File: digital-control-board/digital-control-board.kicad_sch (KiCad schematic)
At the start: 0 parts

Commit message: Get some design from rp minimal board
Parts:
- added C1, C19, C5: 10u, Capacitor_SMD:C_0805_2012Metric, symbol Device:C
- added C10, C9: 4.7u, Capacitor_SMD:C_0402_1005Metric, symbol Device:C
- added C11, C12, C13, C14, C15, C16, C17, C18, C2, C20, C21, C8: 100n, Capacitor_SMD:C_0402_1005Metric, symbol Device:C
- added C22: DNF, Capacitor_SMD:C_0402_1005Metric, symbol Device:C
- added C3, C4: 15p, Capacitor_SMD:C_0402_1005Metric, symbol Device:C
- added C6, C7: 4.7u, RP2350_80QFN_minimal:C_0402_1005Metric_small_pads, symbol Device:C
- added DN1: PM127-2-10-S-4.3, programmable-load-library:HDR-SMD_20P-P1.27-V-F-R2-C10-LS4.8, symbol programmable-load-library:PM127-2-10-S-4.3
- added J1: USB_B_Micro, Connector_USB:USB_Micro-B_Amphenol_10103594-0001LF_Horizontal, symbol Connector:USB_B_Micro
- added J4: SM03B-SRSS-TB, Connector_JST:JST_SH_SM03B-SRSS-TB_1x03-1MP_P1.00mm_Horizontal, symbol Connector_Generic_MountingPin:Conn_01x03_MountingPin
- added L1: 3.3u, RP2350_80QFN_minimal:L_pol_2016, symbol Device:L
- added R1, R11, R13, R9: DNF, Resistor_SMD:R_0402_1005Metric, symbol Device:R
- added R10: 0, Resistor_SMD:R_0402_1005Metric, symbol Device:R
- added R2, R4, R6: 1k, Resistor_SMD:R_0402_1005Metric, symbol Device:R
- added R3: 33, Resistor_SMD:R_0402_1005Metric, symbol Device:R
- added R7, R8: 27, Resistor_SMD:R_0402_1005Metric, symbol Device:R
- added SW1, SW2: SW_Push, Button_Switch_SMD:SW_Push_1P1T_NO_Vertical_Wuerth_434133025816, symbol Switch:SW_Push
- added U1: RP2350_80QFN, RP2350_80QFN_minimal:RP2350-QFN-80-1EP_10x10_P0.4mm_EP3.4x3.4mm_ThermalVias, symbol MCU_RaspberryPi_RP2350:RP2350_80QFN
- added U2: NCP1117-3.3_SOT223, Package_TO_SOT_SMD:SOT-223-3_TabPin2, symbol Regulator_Linear:NCP1117-3.3_SOT223
- added U3: W25Q128JVS, Package_SO:SOIC-8_5.23x5.23mm_P1.27mm, symbol Memory_Flash:W25Q128JVS
- added U4: DNF, Package_SO:SOIC-8_5.23x5.23mm_P1.27mm, symbol Memory_Flash:W25Q128JVS
- added Y1: ABM8-272-T3, Crystal:Crystal_SMD_3225-4Pin_3.2x2.5mm, symbol Device:Crystal_GND24
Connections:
- new net: C4.1, R2.2, Y1.3
- new net: R7.2, U1.67 (USB_DP)
- new net: R8.2, U1.66 (USB_DM)
- new net: R4.1, SW2.1
- new net +1V1: C10.1, C11.1, C7.1, C8.1, L1.1, U1.10 (DVDD), U1.32 (DVDD), U1.51 (DVDD), U1.65 (VREG_FB)
- new net +3V3: C12.1, C13.1, C14.1, C15.1, C16.1, C17.1, C18.1, C19.1, C2.1, C20.1, C21.1, C22.1, C5.1, C6.1, R1.1, R13.1, R3.1, U1.15 (IOVDD), U1.24 (IOVDD), U1.29 (IOVDD), U1.41 (IOVDD), U1.5 (IOVDD), U1.50 (IOVDD), U1.59 (ADC_AVDD), U1.60 (IOVDD), U1.64 (VREG_VIN), U1.68 (USB_OTP_VDD), U1.69 (QSPI_IOVDD), U1.76 (IOVDD), U2.2 (VO), U3.8 (VCC), U4.8 (VCC)
- new net FLASH2_SS: R11.2, R13.2, U4.1 (~{CS})
- new net FLASH_SS: R1.2, R10.2, R9.2, U3.1 (~{CS})
- new net GND: C1.2, C10.2, C11.2, C12.2, C13.2, C14.2, C15.2, C16.2, C17.2, C18.2, C19.2, C2.2, C20.2, C21.2, C22.2, C3.2, C4.2, C5.2, C6.2, C7.2, C8.2, C9.2, J1.5 (GND), J1.6 (Shield), J4.2 (Pin_2), J4.MP (MountPin), R4.2, SW1.1, U1.62 (VREG_PGND), U1.81 (GND), U2.1 (GND), U3.4 (GND), U4.4 (GND), Y1.2, Y1.4
- new net GPIO0: R11.1, U1.77 (GPIO0)
- new net GPIO1: U1.78 (GPIO1)
- new net GPIO10: U1.8 (GPIO10)
- new net GPIO11: U1.9 (GPIO11)
- new net GPIO12: U1.11 (GPIO12)
- new net GPIO13: U1.12 (GPIO13)
- new net GPIO14: U1.13 (GPIO14)
- new net GPIO15: U1.14 (GPIO15)
- new net GPIO16: U1.16 (GPIO16)
- new net GPIO17: U1.17 (GPIO17)
- new net GPIO18: U1.18 (GPIO18)
- new net GPIO19: U1.19 (GPIO19)
- new net GPIO2: U1.79 (GPIO2)
- new net GPIO20: U1.20 (GPIO20)
- new net GPIO21: U1.21 (GPIO21)
- new net GPIO22: U1.22 (GPIO22)
- new net GPIO23: U1.23 (GPIO23)
- new net GPIO24: U1.25 (GPIO24)
- new net GPIO25: U1.26 (GPIO25)
- new net GPIO26: U1.27 (GPIO26)
- new net GPIO27: U1.28 (GPIO27)
- new net GPIO28: U1.36 (GPIO28)
- new net GPIO29: U1.37 (GPIO29)
- new net GPIO3: U1.80 (GPIO3)
- new net GPIO30: U1.38 (GPIO30)
- new net GPIO31: U1.39 (GPIO31)
- new net GPIO32: U1.40 (GPIO32)
- new net GPIO33: U1.42 (GPIO33)
- new net GPIO34: U1.43 (GPIO34)
- new net GPIO35: U1.44 (GPIO35)
- new net GPIO36: U1.45 (GPIO36)
- new net GPIO37: U1.46 (GPIO37)
- new net GPIO38: U1.47 (GPIO38)
- new net GPIO39: U1.48 (GPIO39)
- new net GPIO4: U1.1 (GPIO4)
- new net GPIO40_ADC0: U1.49 (GPIO40_ADC0)
- new net GPIO41_ADC1: U1.52 (GPIO41_ADC1)
- new net GPIO42_ADC2: U1.53 (GPIO42_ADC2)
- new net GPIO43_ADC3: U1.54 (GPIO43_ADC3)
- new net GPIO44_ADC4: U1.55 (GPIO44_ADC4)
- new net GPIO45_ADC5: U1.56 (GPIO45_ADC5)
- new net GPIO46_ADC6: U1.57 (GPIO46_ADC6)
- new net GPIO47_ADC7: U1.58 (GPIO47_ADC7)
- new net GPIO5: U1.2 (GPIO5)
- new net GPIO6: U1.3 (GPIO6)
- new net GPIO7: U1.4 (GPIO7)
- new net GPIO8: U1.6 (GPIO8)
- new net GPIO9: U1.7 (GPIO9)
- new net QSPI_SCLK: U1.71 (QSPI_SCLK), U3.6 (CLK), U4.6 (CLK)
- new net QSPI_SD0: U1.72 (QSPI_SD0), U3.5 (DI(IO0)), U4.5 (DI(IO0))
- new net QSPI_SD1: U1.74 (QSPI_SD1), U3.2 (DO(IO1)), U4.2 (DO(IO1))
- new net QSPI_SD2: U1.73 (QSPI_SD2), U3.3 (IO2), U4.3 (IO2)
- new net QSPI_SD3: U1.70 (QSPI_SD3), U3.7 (IO3), U4.7 (IO3)
- new net QSPI_SS: R6.1, U1.75 (QSPI_SS)
- new net RUN: SW2.2, U1.35 (RUN)
- new net SWCLK: J4.1 (Pin_1), U1.33 (SWCLK)
- new net SWD: J4.3 (Pin_3), U1.34 (SWD)
- new net USB_D+: J1.3 (D+), R7.1
- new net USB_D-: J1.2 (D-), R8.1
- new net VBUS: C1.1, J1.1 (VBUS), U2.3 (VI)
- new net VREG_AVDD: C9.1, R3.2, U1.61 (VREG_AVDD)
- new net VREG_LX: L1.2, U1.63 (VREG_LX)
- new net XIN: C3.1, U1.30 (XIN), Y1.1
- new net XOUT: R2.1, U1.31 (XOUT)
- new net ~{USB_BOOT}: R6.2, SW1.2
- no-connect marks 0 -> 1
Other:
- note added: "12MHz Crystal"
- note added: "JST Debug Connector"
- note added: "Make sure R7 and R8 are close to RP2350"
- note added: "Optional Secondary flash or PSRAM (U4), using the second chip select (XIP_SS_N[1]) on GPIO0. N.B. Pull-up R13 will be required as GPIOs default to pull-downs at power-up."
- note added: "Power"
- note added: "Primary Flash"
- note added: "Reference the RP2350 minimal design example caz I'm lazy"
- note added: "Secondary Flash/PSRAM"

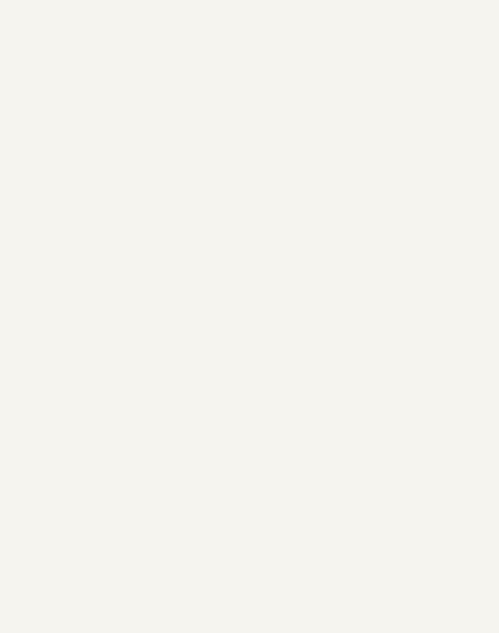
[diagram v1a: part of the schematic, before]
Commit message: Update sch
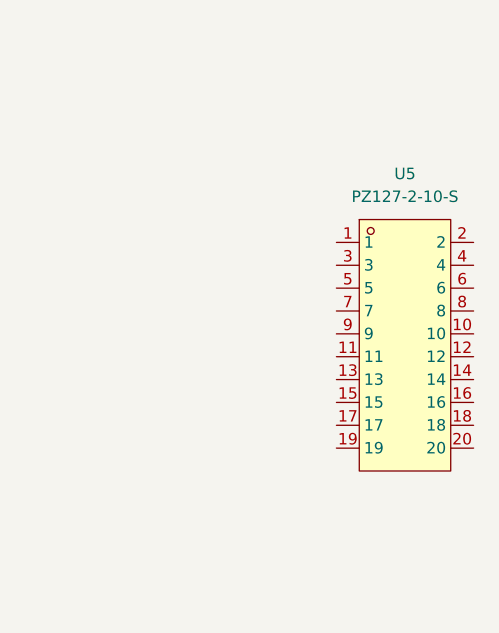
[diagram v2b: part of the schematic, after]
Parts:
- added U5: PZ127-2-10-S, programmable-load-library:HDR-SMD_PZ127-2-10-S, symbol programmable-load-library:PZ127-2-10-S
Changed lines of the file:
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@@
+	)
+	(symbol
+		(lib_id "programmable-load-library:PZ127-2-10-S")
+		(at 519.43 64.77 0)
+		(unit 1)
+		(exclude_from_sim no)
+		(in_bom yes)
+		(on_board yes)
+		(dnp no)
+		(fields_autoplaced yes)
+		(property "Reference" "U5"
+			(at 519.43 45.72 0)
+			(effects
+				(font
+					(size 1.27 1.27)
+				)
+			)
+		)
+		(property "Value" "PZ127-2-10-S"
+			(at 519.43 48.26 0)
+			(effects
+				(font
+					(size 1.27 1.27)
+				)
+			)
+		)
+		(property "Footprint" "programmable-load-library:HDR-SMD_PZ127-2-10-S"
+			(at 519.43 83.82 0)
+			(effects
+				(font
+					(size 1.27 1.27)
+				)
+				(hide yes)
+			)
+		)
+		(property "Datasheet" ""
+			(at 519.43 64.77 0)
+			(effects
+				(font
+					(size 1.27 1.27)
+				)
+				(hide yes)
+			)
+		)
+		(property "Description" ""
+			(at 519.43 64.77 0)
+			(effects
+				(font
+					(size 1.27 1.27)
+				)
+				(hide yes)
+			)
+		)
+		(property "LCSC Part" "C3975193"
+			(at 519.43 86.36 0)
+			(effects
+				(font
+					(size 1.27 1.27)
+				)
+				(hide yes)
+			)
+		)
+		(pin "19"
+		)
+		(pin "2"
+		)
+		(pin "4"
+		)
+		(pin "6"
+		)
+		(pin "8"
+		)
+		(pin "10"
+		)
+		(pin "12"
+		)
+		(pin "14"
+		)
+		(pin "16"
+		)
+		(pin "18"
+		)
+		(pin "20"
+		)
+		(pin "7"
+		)
+		(pin "9"
+		)
+		(pin "11"
+		)
+		(pin "13"
+		)
+		(pin "15"
+		)
+		(pin "17"
+		)
+		(pin "1"
+		)
+		(pin "3"
+		)
+		(pin "5"
+		)
+		(instances
+			(project ""
+				(path "/8554ec12-f084-4452-82fa-ded977d90d56"
+					(reference "U5")
+					(unit 1)
+				)
+			)
+		)
 	)
 	(symbol

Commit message: Update digital-control-board
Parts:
- removed DN1: PM127-2-10-S-4.3, programmable-load-library:HDR-SMD_20P-P1.27-V-F-R2-C10-LS4.8, symbol programmable-load-library:PM127-2-10-S-4.3
- removed U5: PZ127-2-10-S, programmable-load-library:HDR-SMD_PZ127-2-10-S, symbol programmable-load-library:PZ127-2-10-S
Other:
- added sheet analog_interface (analog_interface.kicad_sch)
- moved on the sheet: C1, C10, C11, C12, C13, C14, C15, C16, C17, C18, C19, C2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

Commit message: Add ADC input filter
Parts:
- removed C22: DNF, Capacitor_SMD:C_0402_1005Metric, symbol Device:C
- removed J1: USB_B_Micro, Connector_USB:USB_Micro-B_Amphenol_10103594-0001LF_Horizontal, symbol Connector:USB_B_Micro
- removed R11, R13: DNF, Resistor_SMD:R_0402_1005Metric, symbol Device:R
- removed U4: DNF, Package_SO:SOIC-8_5.23x5.23mm_P1.27mm, symbol Memory_Flash:W25Q128JVS
- added C37: 2.2n, Capacitor_SMD:C_0603_1608Metric, symbol Device:C
- added R15, R16: 5.1k, Resistor_SMD:R_0603_1608Metric, symbol Device:R_Small
- added R17: 1M, Resistor_SMD:R_0603_1608Metric, symbol Device:R
- added USB1: TYPE-C 16PIN 2MD(073), programmable-load-library:USB-C-SMD_TYPE-C-6PIN-2MD-073, symbol programmable-load-library:TYPE-C16PIN2MD(073)
- C10, C11, C12, C13, C14, C15, C16, C17, C18, C2, C20, C21, C3, C4, C8, C9: footprint Capacitor_SMD:C_0402_1005Metric -> Capacitor_SMD:C_0603_1608Metric
- C6, C7: footprint RP2350_80QFN_minimal:C_0402_1005Metric_small_pads -> Capacitor_SMD:C_0603_1608Metric
- R1, R10, R2, R3, R4, R6, R7, R8, R9: footprint Resistor_SMD:R_0402_1005Metric -> Resistor_SMD:R_0603_1608Metric
- U1: footprint RP2350_80QFN_minimal:RP2350-QFN-80-1EP_10x10_P0.4mm_EP3.4x3.4mm_ThermalVias -> Package_DFN_QFN:QFN-80-1EP_10x10mm_P0.4mm_EP3.4x3.4mm
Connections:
- net GND: now also C37.2, R17.2, USB1.1 (GND), USB1.12 (GND)
- net USB_D+: now also USB1.6 (DP1), USB1.8 (DP2)
- net USB_D-: now also USB1.5 (DN2), USB1.7 (DN1)
- net VBUS: now also USB1.11 (VBUS), USB1.2 (VBUS)
- new net: R16.1, USB1.10 (CC2)
- new net: R15.1, USB1.4 (CC1)
- new net Earth: C37.1, R17.1, USB1.13 (SHELL), USB1.14 (SHELL)
- no-connect marks 1 -> 0
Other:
- added sheet connector (connector.kicad_sch)
- added sheet mosfet_gate_interface (mosfet_gate_interface.kicad_sch)
- note removed: "Optional Secondary flash or PSRAM (U4), using the second chip select (XIP_SS_N[1]) on GPIO0. N.B. Pull-up R13 will be required as GPIOs default to pull-downs at power-up."
- note removed: "Secondary Flash/PSRAM"
- moved on the sheet: C1, C2, C3, C4, C5, R1, R10, R2, R9, U2, U3, Y1
